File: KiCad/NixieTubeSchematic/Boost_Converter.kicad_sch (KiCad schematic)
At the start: 33 parts

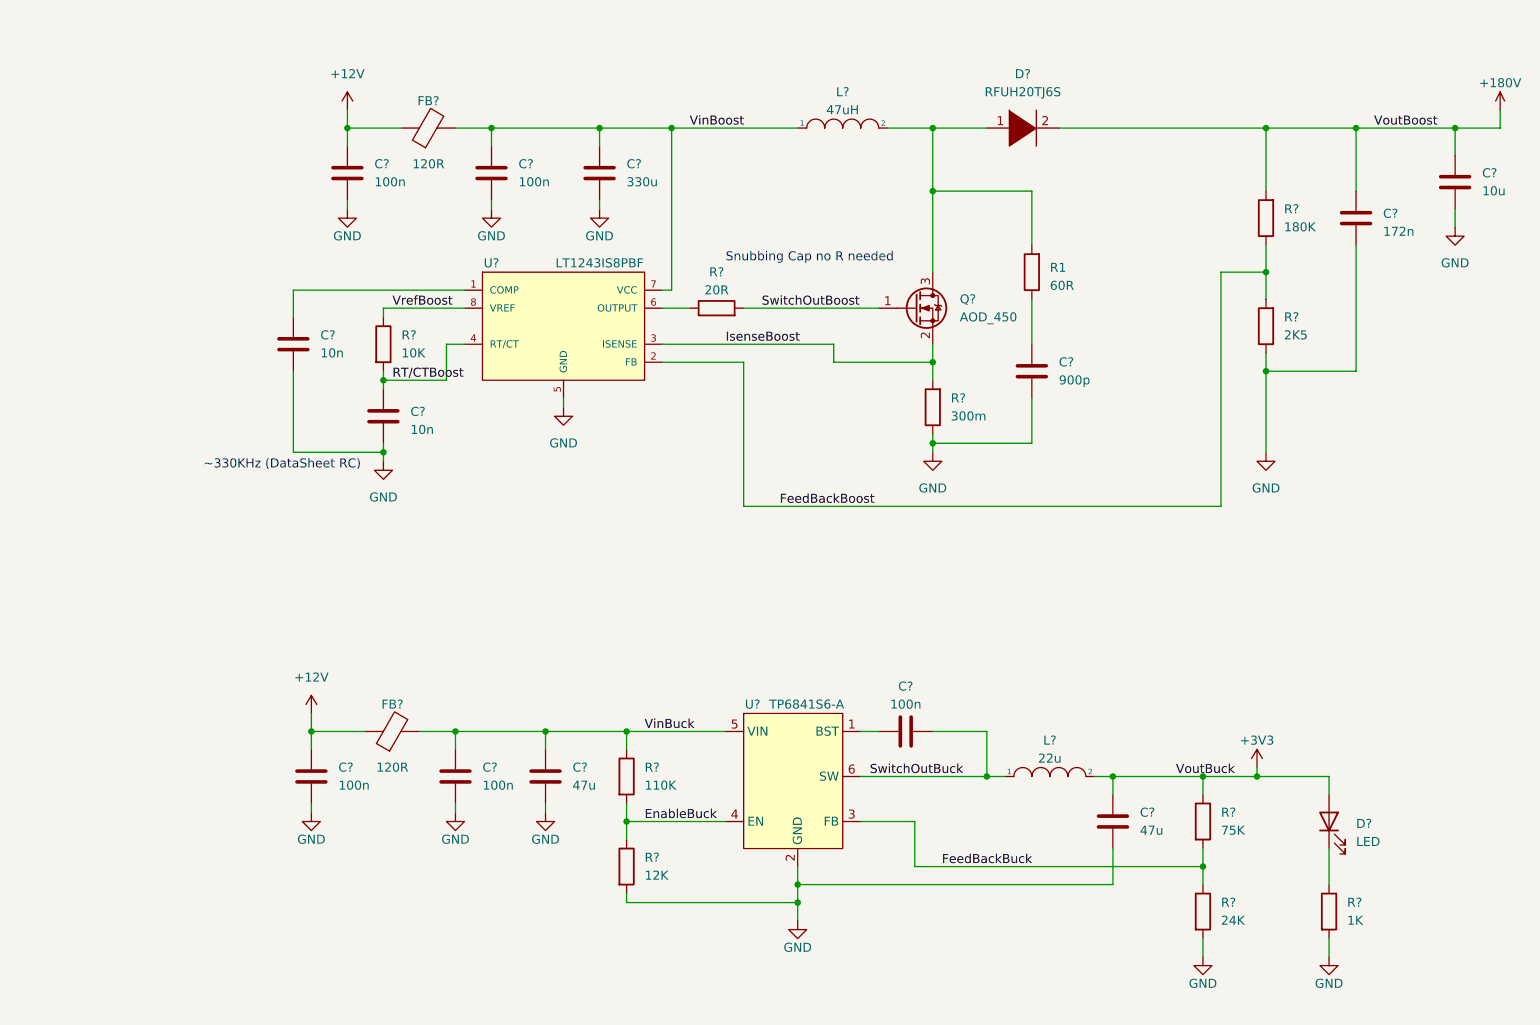
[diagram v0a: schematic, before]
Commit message: Small changes
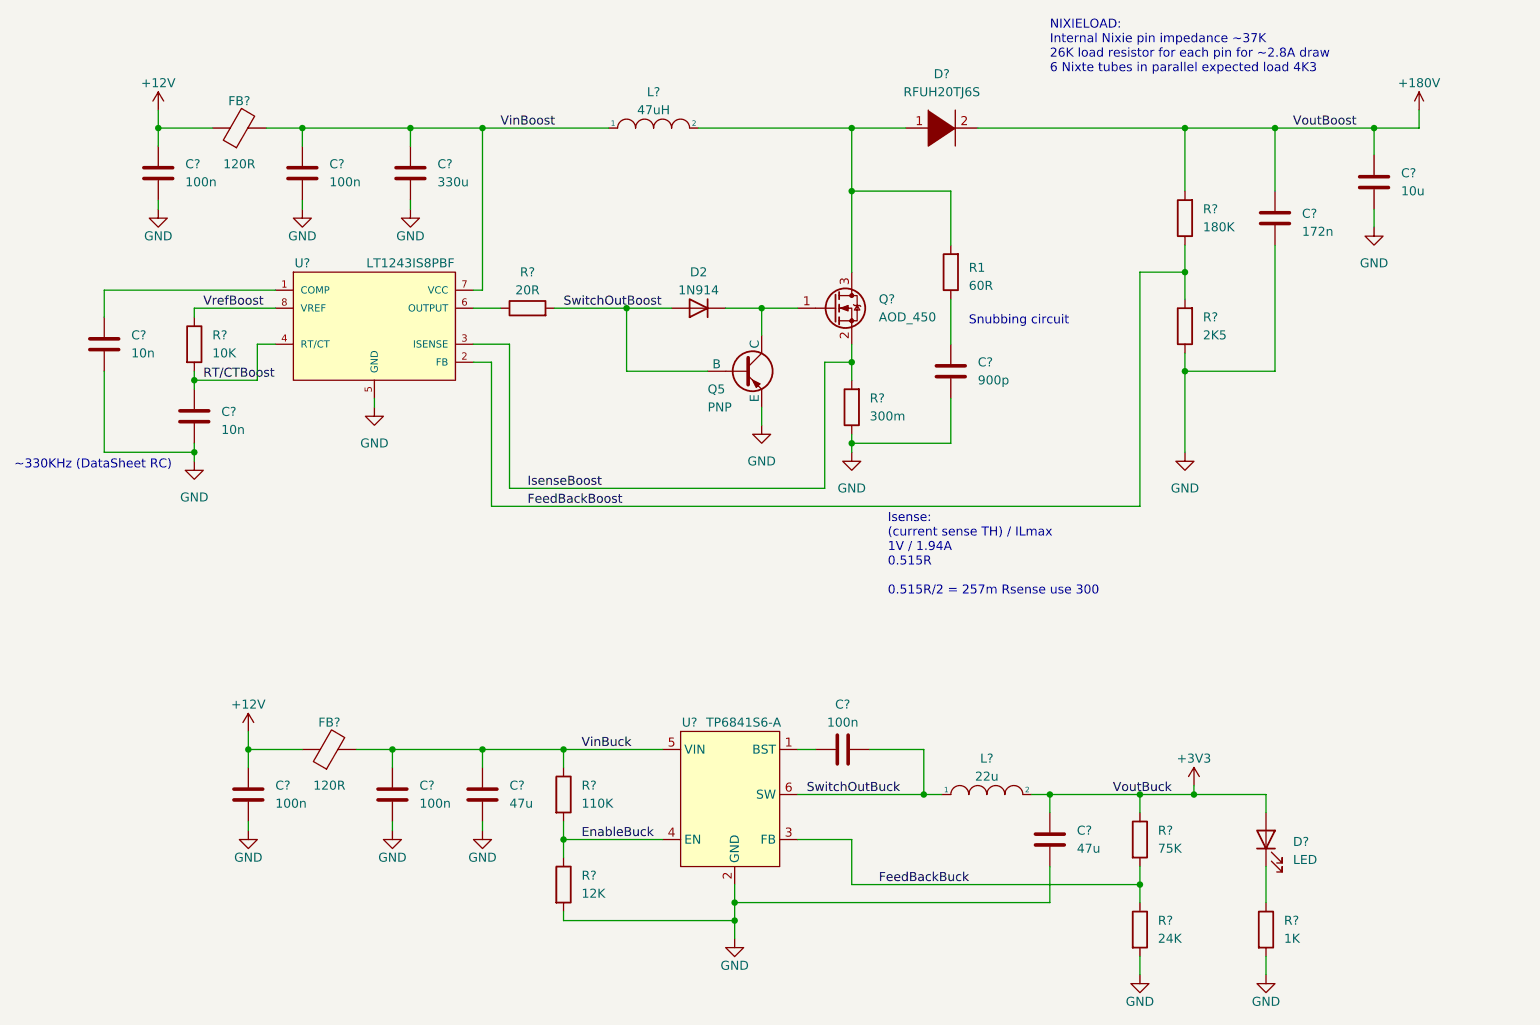
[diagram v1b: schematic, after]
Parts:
- added D2: 1N914, Diode_THT:D_DO-35_SOD27_P7.62mm_Horizontal, symbol Diode:1N914
- added Q5: PNP, symbol Simulation_SPICE:PNP
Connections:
- net GND: now also Q5.3 (E)
- net SwitchOutBoost: now also D2.2 (A), Q5.2 (B); no longer Q?.1 (G)
- new net: D2.1 (K), Q5.1 (C), Q?.1 (G)
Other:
- note added: "Isense: (current sense TH) / ILmax 1V / 1.94A 0.515R 0.515R/2 = 257m Rsense use 300"
- note added: "NIXIELOAD: Internal Nixie pin impedance ~37K 26K load resistor for each pin for ~2.8A draw 6 Nixte tubes in parallel expected load 4K3"
- note added: "Snubbing circuit"
- note removed: "Snubbing Cap no R needed"
- moved on the sheet: C?, D?, FB?, L?, Q?, R1, R?, U?
